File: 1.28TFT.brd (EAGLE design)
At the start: 12 parts, among them M1 LCD_FPCST

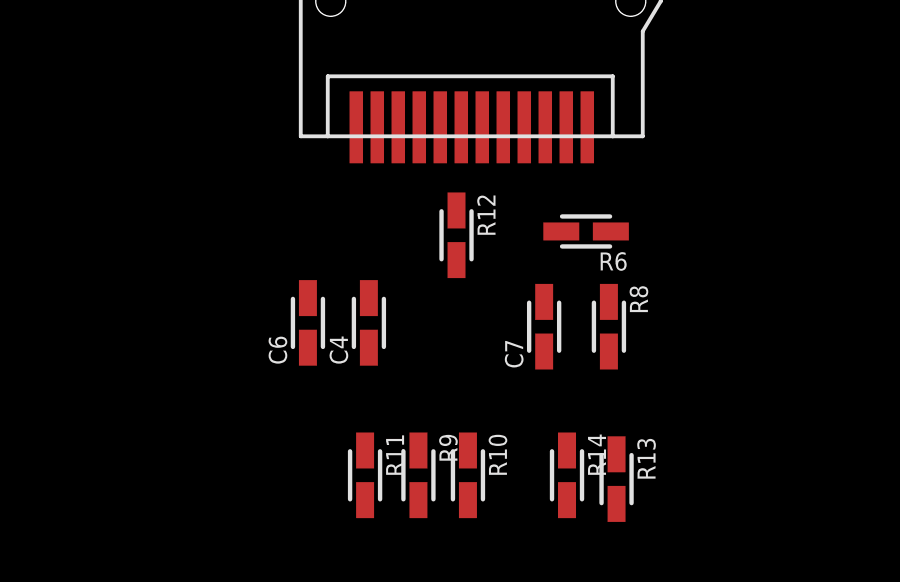
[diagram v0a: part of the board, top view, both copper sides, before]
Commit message: bugfix
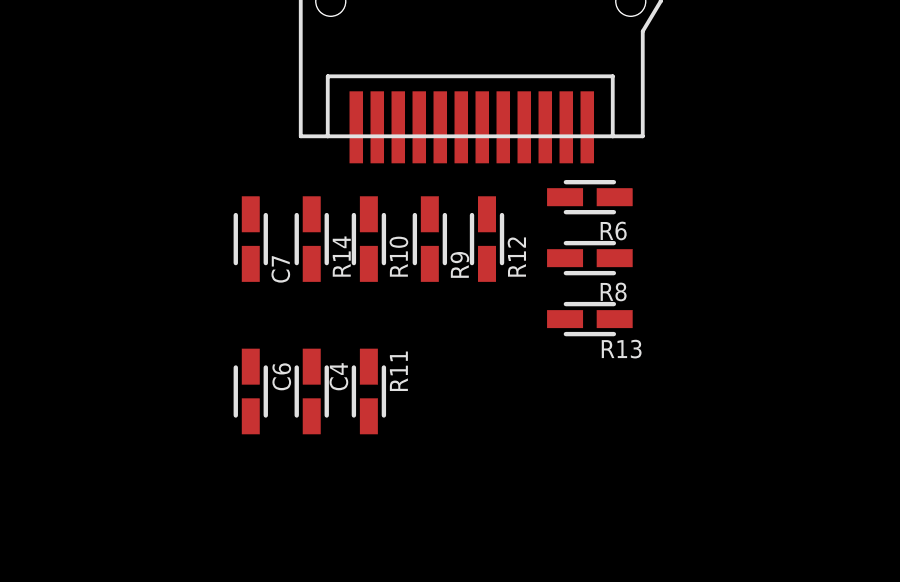
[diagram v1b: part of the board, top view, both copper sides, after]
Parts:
- C6, C7: value 0.1u -> 0.1uF
- R10, R12, R13, R9: value 1k -> 1K
- R11: value 10k -> 10K
- R8: value 51k -> 51K
- moved R14 11.6 mm to (5.59, 17.3)
- moved C7 10.2 mm to (3.56, 17.3), turned to 270 degrees
- moved R10 8.54 mm to (7.49, 17.3)
- moved R9 7.88 mm to (9.53, 17.3)
- moved R13 5.41 mm to (14.9, 14.6), turned to 0 degrees
- moved C4 2.98 mm to (5.59, 12.2)
- moved C6 2.98 mm to (3.56, 12.2)
- moved R11 2.80 mm to (7.49, 12.2)
- moved R8 2.37 mm to (14.9, 16.6), turned to 180 degrees
- moved R6 1.15 mm to (14.9, 18.7)
- moved R12 1.02 mm to (11.4, 17.3)
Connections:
- net DC renamed N$5
- new net N$4: M1.10, R10.P$1
- net SDA: no longer M1.10, R10.P$1
